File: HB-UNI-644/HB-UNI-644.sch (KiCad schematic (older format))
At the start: 49 parts, among them J1 FTDI, J10 ICSP, J11 RAW, J12 Conn_Gnd, J13 Conn_NTC, J2 GS2, J3 I2C_1, J4 GS2, J5 I2C_2, J6 I2C_3, J7 I2C_4, J8 Conn_A, J9 Conn_B, Q1 IRLML6244/IRLML0030, SW1 CONFIG, U1 ATMEGA644PA-AU, U2 CC1101, U3 MAX1724, U4 LM3480-3.3, Y1 8MHz

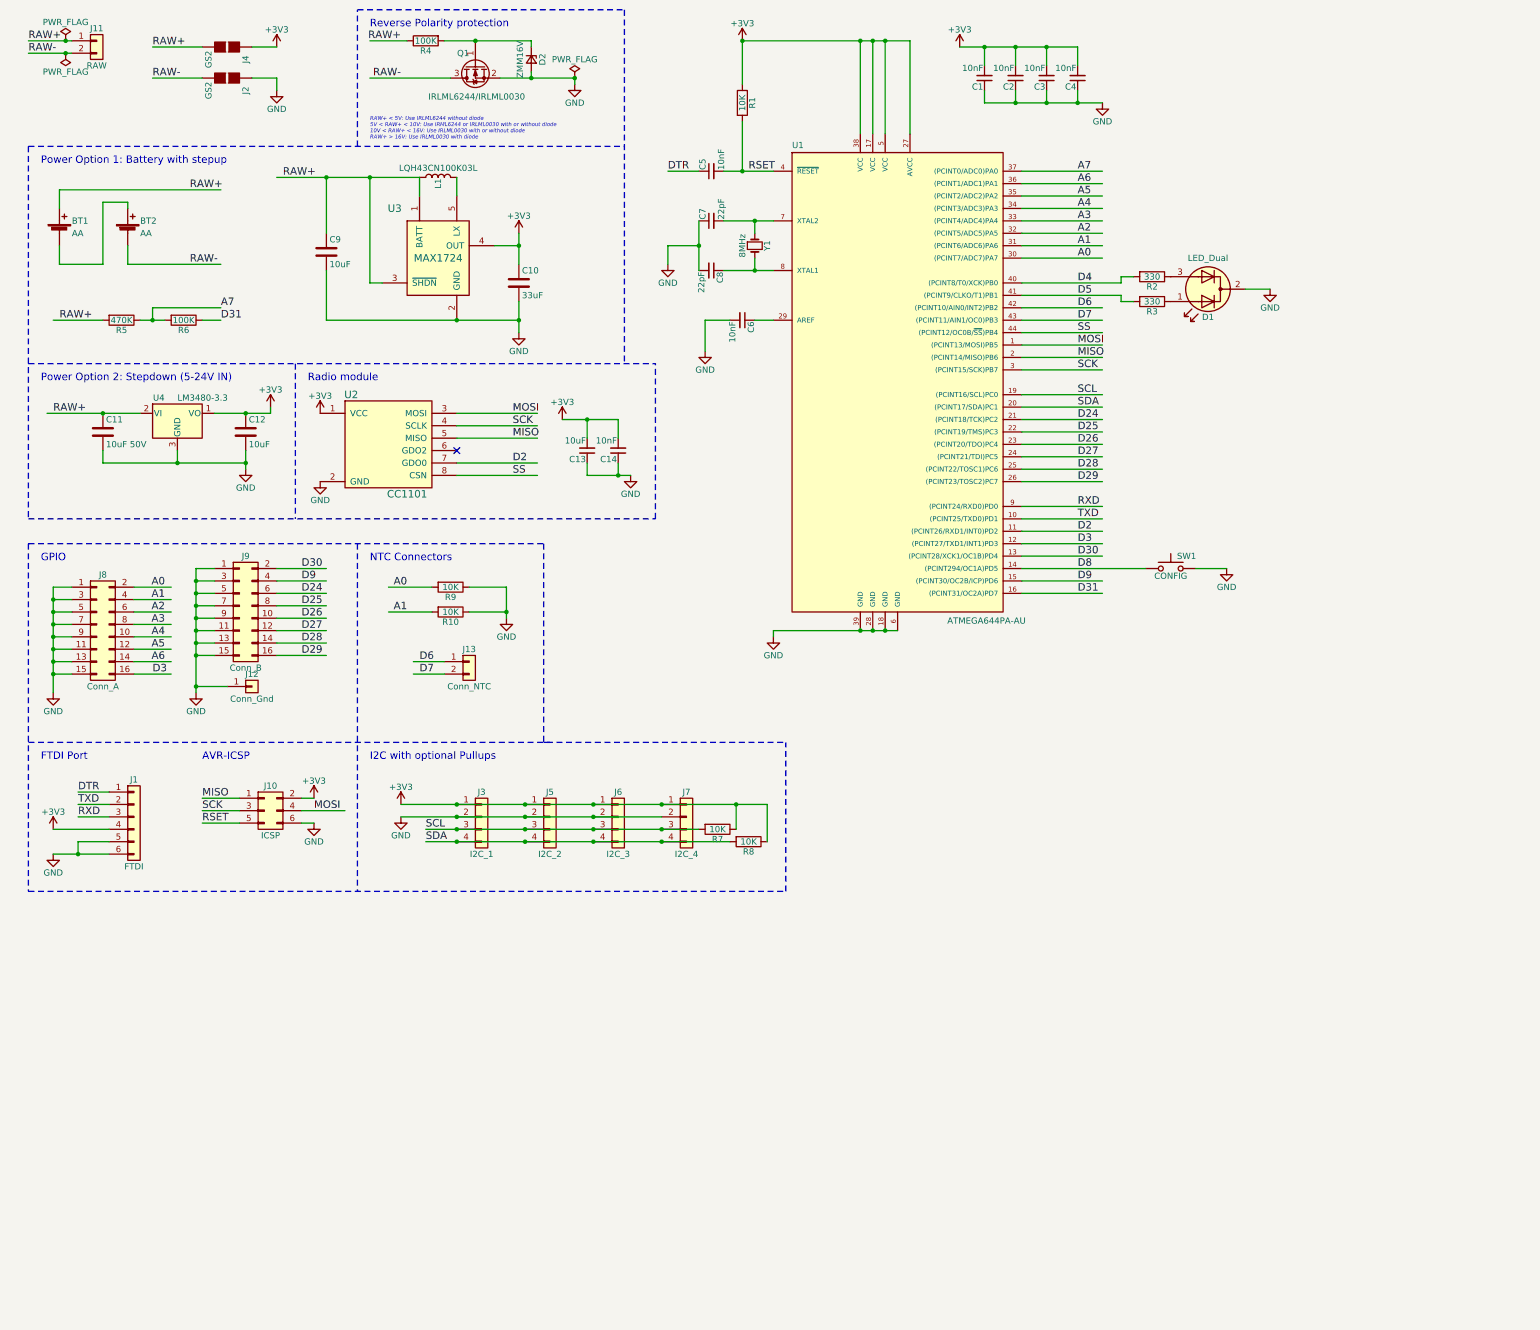
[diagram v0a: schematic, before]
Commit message: Revision 2 of HB-UNI-644
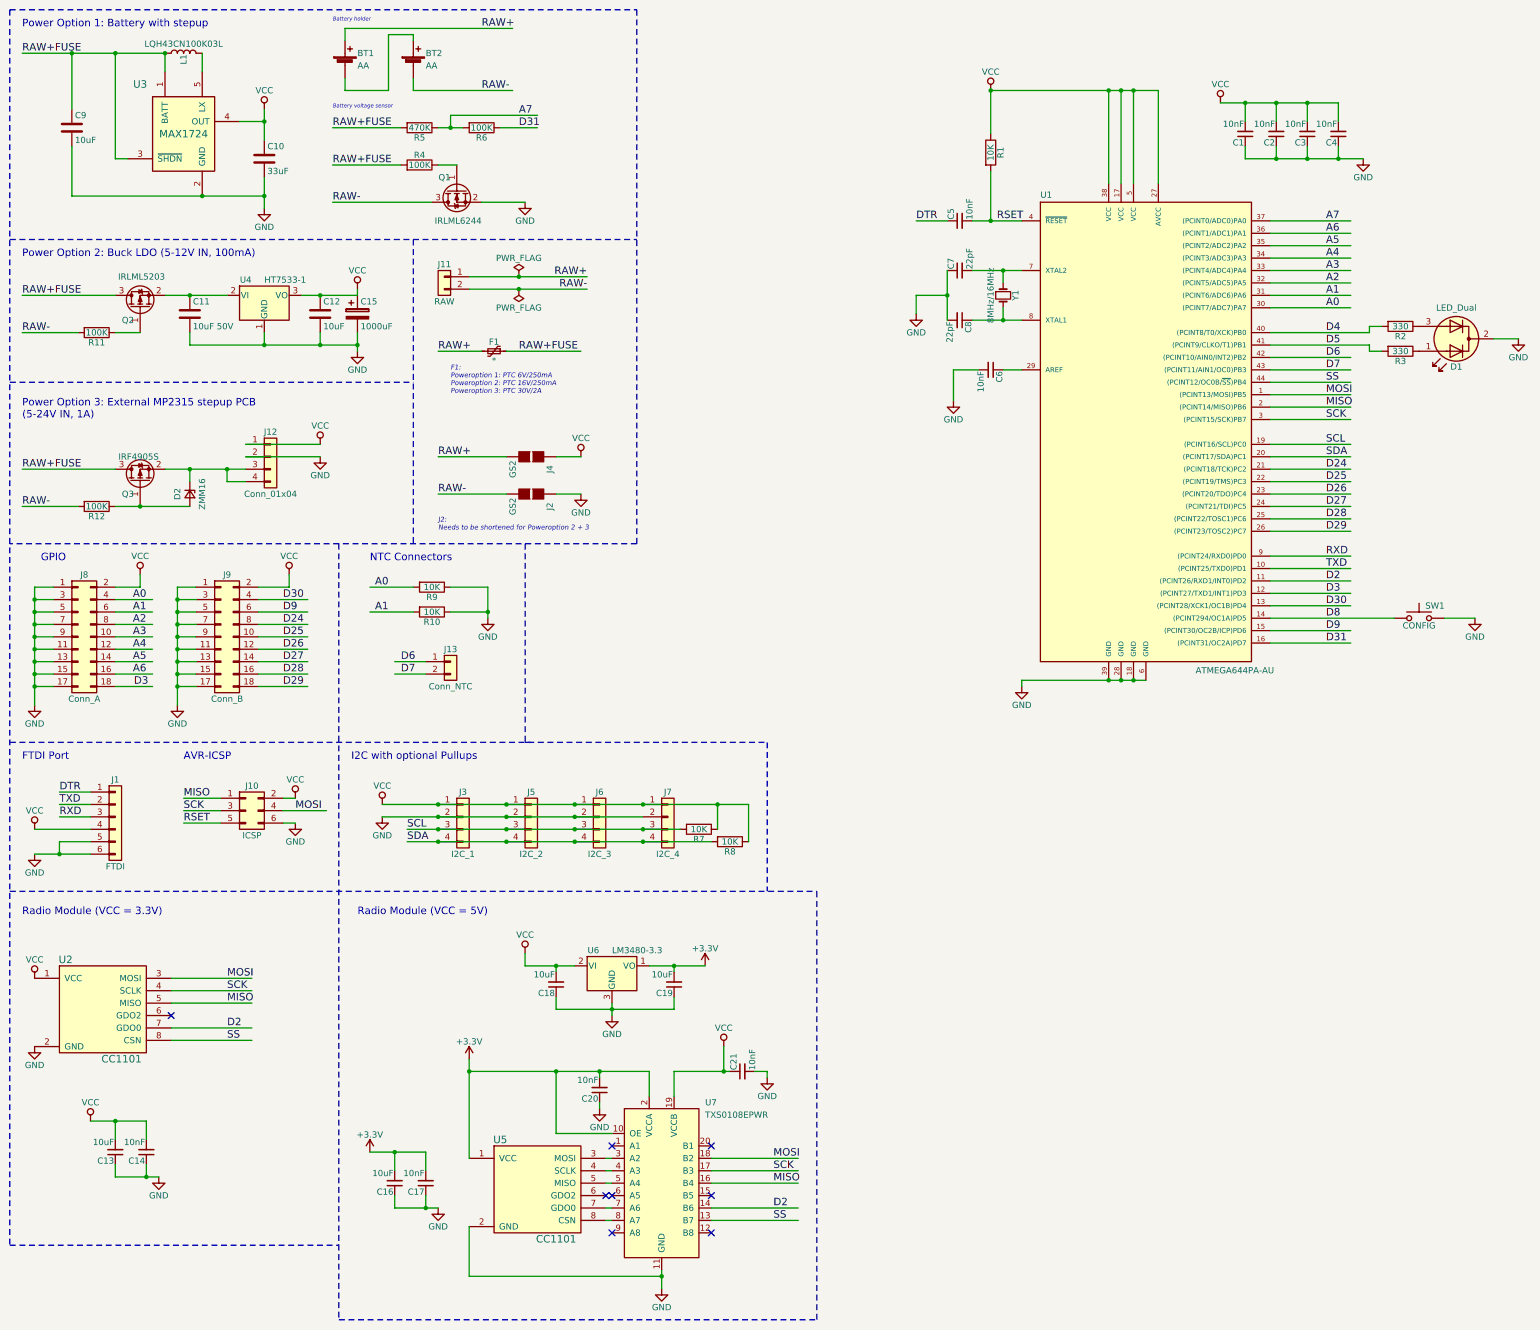
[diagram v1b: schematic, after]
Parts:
- removed J12: Conn_Gnd, Pin_Headers:Pin_Header_Straight_1x01_Pitch2.54mm, symbol Conn_01x01
- removed J8: Conn_A, Pin_Headers:Pin_Header_Straight_2x08_Pitch2.54mm, symbol Conn_02x08_Odd_Even
- removed J9: Conn_B, Pin_Headers:Pin_Header_Straight_2x08_Pitch2.54mm, symbol Conn_02x08_Odd_Even
- removed U4: LM3480-3.3, TO_SOT_Packages_SMD:SOT-23_Handsoldering, symbol LM3480-3.3
- added C15: 1000uF, Capacitors_THT:CP_Radial_D8.0mm_P3.50mm, symbol CP
- added C16, C18, C19: 10uF, Capacitors_SMD:C_0805_HandSoldering, symbol C_Small
- added C17, C20, C21: 10nF, Capacitors_SMD:C_0805_HandSoldering, symbol C_Small
- added F1: *, Resistors_SMD:R_1206_HandSoldering, symbol Polyfuse_Small
- added J12: Conn_01x04, Pin_Headers:Pin_Header_Straight_1x04_Pitch2.54mm, symbol Conn_01x04
- added J8: Conn_A, Pin_Headers:Pin_Header_Straight_2x09_Pitch2.54mm, symbol Conn_02x09_Odd_Even
- added J9: Conn_B, Pin_Headers:Pin_Header_Straight_2x09_Pitch2.54mm, symbol Conn_02x09_Odd_Even
- added Q2: IRLML5203, TO_SOT_Packages_SMD:SOT-23_Handsoldering, symbol Q_PMOS_GSD
- added Q3: IRF4905S, TO_SOT_Packages_SMD:TO-263-2, symbol Q_PMOS_GSD
- added R11, R12: 100K, Resistors_SMD:R_0805_HandSoldering, symbol R
- added U4: HT7533-1, TO_SOT_Packages_SMD:SOT-89-3_Handsoldering, symbol HT7533-1
- added U5: CC1101, Homebrew:CC1101, symbol CC1101
- added U6: LM3480-3.3, TO_SOT_Packages_SMD:SOT-23, symbol LM3480-3.3
- added U7: TXS0108EPWR, Housings_SSOP:TSSOP-20_4.4x6.5mm_Pitch0.65mm, symbol TXS0108EPWR
- C12, C9: footprint Capacitors_SMD:C_1206_HandSoldering -> Capacitors_SMD:C_0805_HandSoldering
- D2: value ZMM16V -> ZMM16
- Q1: value IRLML6244/IRLML0030 -> IRLML6244
- Y1: value 8MHz -> 8MHz/16MHz
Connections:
- net labels added: +3.3V, RAW+FUSE, VCC
- net labels removed: +3V3
- wire segments 187 -> 243
- no-connect marks 1 -> 8
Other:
- note added: "Battery holder"
- note added: "Battery voltage sensor"
- note added: "F1:\nPoweroption 1: PTC 6V/250mA\nPoweroption 2: PTC 16V/250mA\nPoweroption 3: PTC 30V/2A"
- note added: "J2:\nNeeds to be shortened for Poweroption 2 + 3"
- note added: "Power Option 2: Buck LDO (5-12V IN, 100mA)"
- note added: "Power Option 3: External MP2315 stepup PCB\n(5-24V IN, 1A)"
- note added: "Radio Module (VCC = 3.3V)"
- note added: "Radio Module (VCC = 5V)"
- note removed: "Power Option 2: Stepdown (5-24V IN)"
- note removed: "RAW+ < 5V: Use IRLML6244 without diode\n5V < RAW+ < 10V: Use IRML6244 or IRLML0030 with or without diode\n10V < RAW+ < 16V: Use IRLML0030 with or without diode\nRAW+ > 16V: Use IRLML0030 with diode"
- note removed: "Radio module"
- note removed: "Reverse Polarity protection"
- moved on the sheet: BT1, BT2, C1, C10, C11, C12, C13, C14, C2, C3, C4, C5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
